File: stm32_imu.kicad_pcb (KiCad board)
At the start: 4 copper layers, 27.5 x 41 mm, 43 parts, among them J1 USB_C_Receptacle_USB2.0_16P, J3 TC2030, U1 NRF24L01, U2 USBLC6-2SC6, U3 LM1117MP-3.3, U4 2.4GHz, U5 ICM-20948, U6 STM32F411CEUx, Y1 16MHz, Y2 24MHz

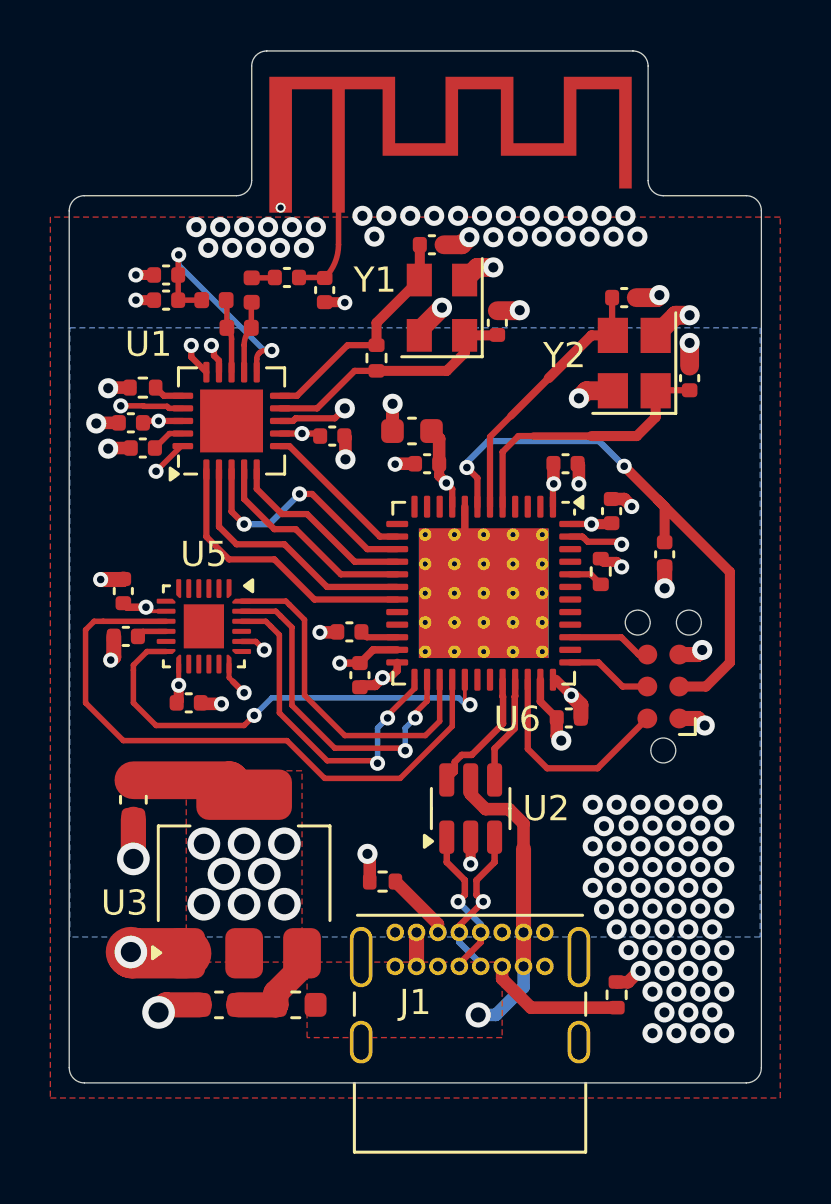
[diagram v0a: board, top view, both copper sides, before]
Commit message: edited layout
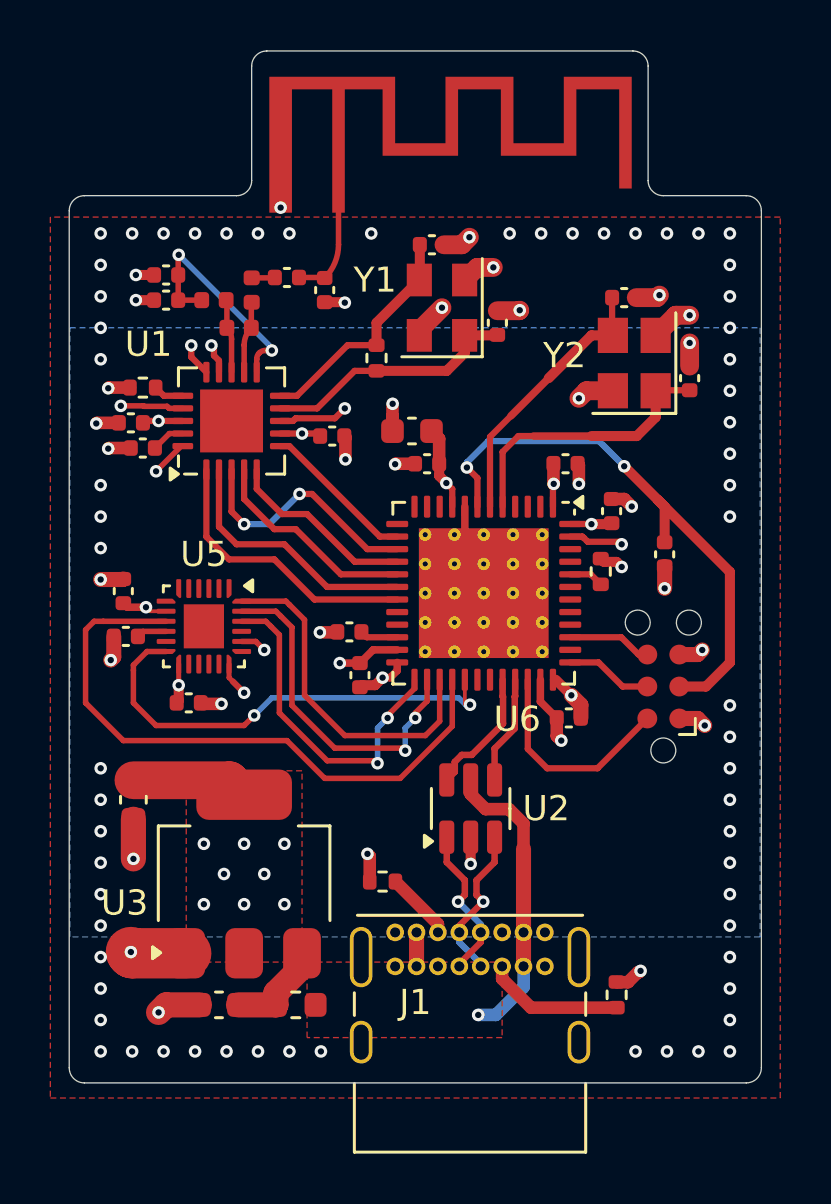
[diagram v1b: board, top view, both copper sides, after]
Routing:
- net GND: vias 133 -> 106
